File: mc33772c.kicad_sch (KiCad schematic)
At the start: 11 parts, among them U2 MC33772CTP1AE

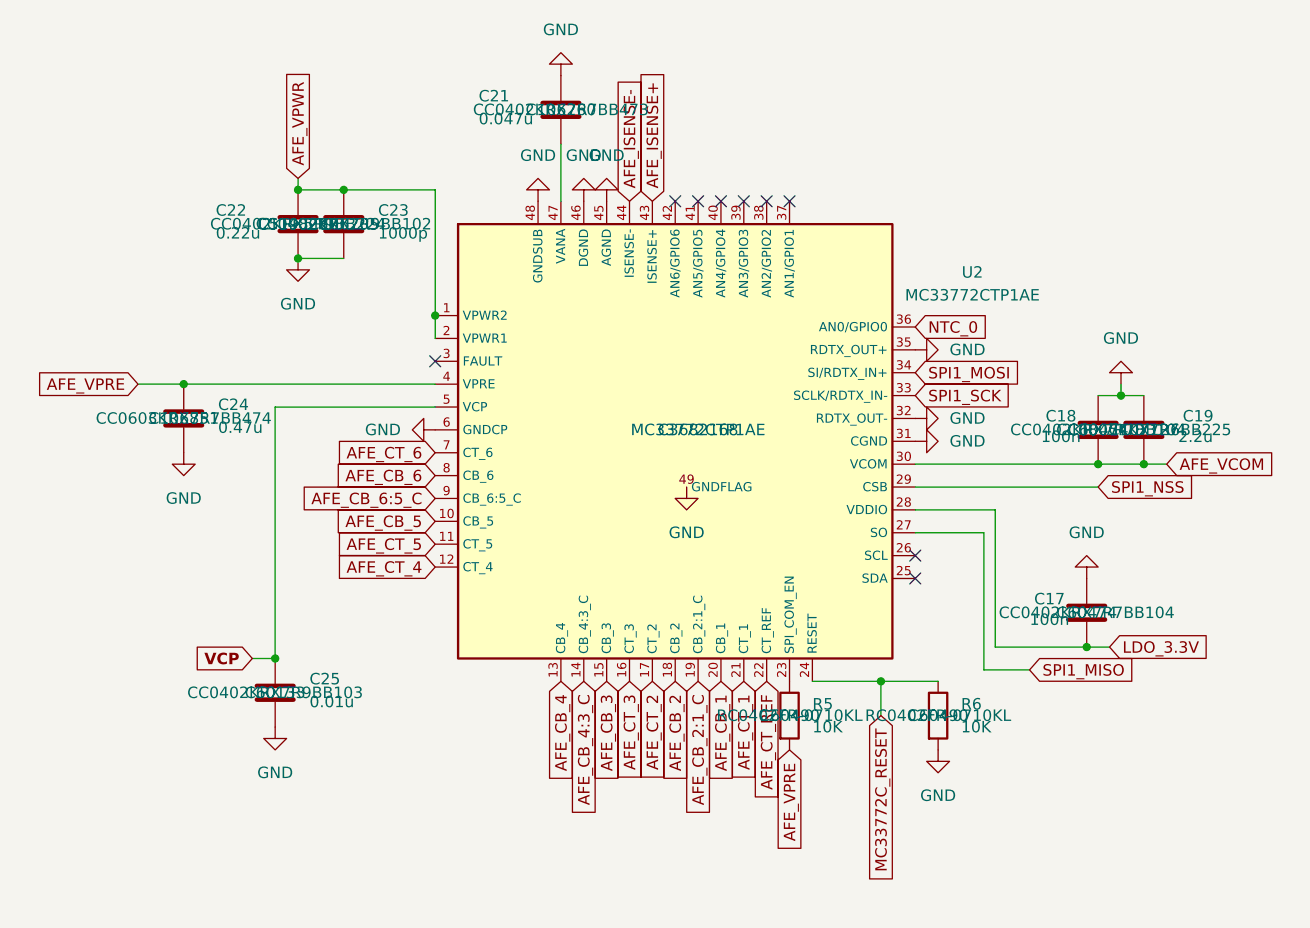
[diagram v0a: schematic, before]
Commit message: shrink, SWD
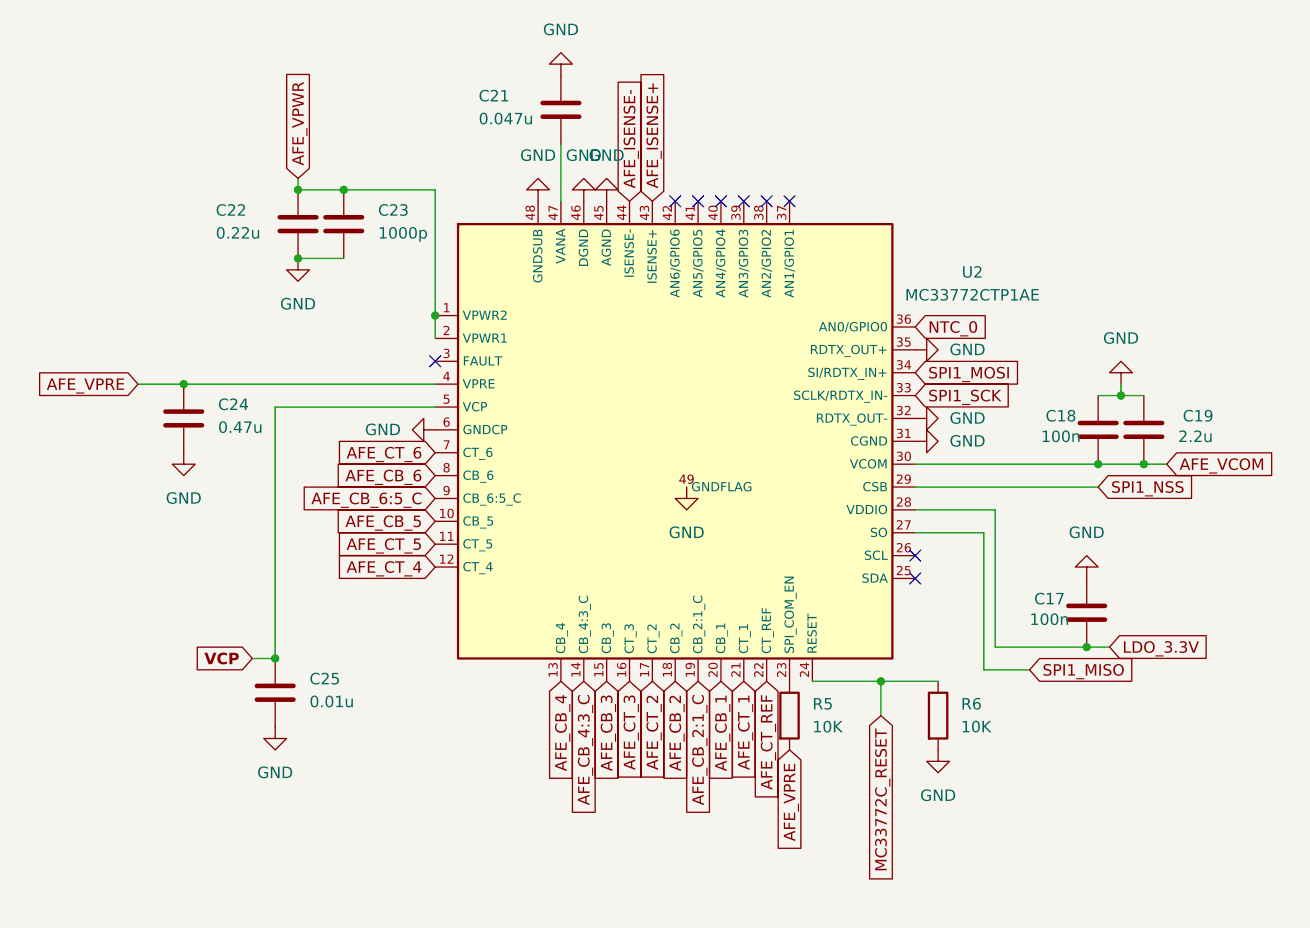
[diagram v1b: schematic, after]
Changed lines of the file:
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@@
 		(property "LCSC Part #" ""
 			(at 140.97 58.42 0)
+			(hide yes)
 			(show_name no)
 			(do_not_autoplace no)
@@
 		(property "MPN" ""
 			(at 140.97 58.42 180)
+			(hide yes)
 			(show_name no)
 			(do_not_autoplace no)
@@
 		(property "LCSC Part #" ""
 			(at 175.26 74.93 0)
+			(hide yes)
 			(show_name no)
 			(do_not_autoplace no)
@@
 		(property "MPN" ""
 			(at 175.26 74.93 90)
+			(hide yes)
 			(show_name no)
 			(do_not_autoplace no)
@@
 		(property "LCSC Part #" "C107127"
 			(at 200.66 83.82 0)
+			(hide yes)
 			(show_name no)
 			(do_not_autoplace no)
@@
 		(property "MPN" "CC0805KKX7R6BB225"
 			(at 200.66 83.82 0)
+			(hide yes)
 			(show_name no)
 			(do_not_autoplace no)
@@
 		(property "LCSC Part #" "C106851"
 			(at 93.98 82.55 0)
+			(hide yes)
 			(show_name no)
 			(do_not_autoplace no)
@@
 		(property "MPN" "CC0603KRX7R7BB474"
 			(at 93.98 82.55 0)
+			(hide yes)
 			(show_name no)
 			(do_not_autoplace no)
@@
 		(property "LCSC Part #" ""
 			(at 104.14 116.84 0)
+			(hide yes)
 			(show_name no)
 			(do_not_autoplace no)
@@
 		(property "MPN" ""
 			(at 104.14 116.84 0)
+			(hide yes)
 			(show_name no)
 			(do_not_autoplace no)
@@
 		(property "LCSC Part #" "C60490"
 			(at 177.8 115.57 0)
+			(hide yes)
 			(show_name no)
 			(do_not_autoplace no)
@@
 		(property "MPN" "RC0402FR-0710KL"
 			(at 177.8 115.57 0)
+			(hide yes)
 			(show_name no)
 			(do_not_autoplace no)
@@
 		(property "LCSC Part #" "C5198287"
 			(at 106.68 60.96 0)
+			(hide yes)
 			(show_name no)
 			(do_not_autoplace no)
@@
 		(property "MPN" "CC0402KRX5R9BB224"
 			(at 106.68 60.96 0)
+			(hide yes)
 			(show_name no)
 			(do_not_autoplace no)
@@
 		(property "LCSC Part #" "C60133"
 			(at 104.14 113.03 0)
+			(hide yes)
 			(show_name no)
 			(do_not_autoplace no)
@@
 		(property "MPN" "CC0402KRX7R9BB103"
 			(at 104.14 113.03 0)
+			(hide yes)
 			(show_name no)
 			(do_not_autoplace no)
@@
 		(property "LCSC Part #" ""
 			(at 106.68 64.77 0)
+			(hide yes)
 			(show_name no)
 			(do_not_autoplace no)
@@
 		(property "MPN" ""
 			(at 106.68 64.77 0)
+			(hide yes)
 			(show_name no)
 			(do_not_autoplace no)
@@
 		(property "LCSC Part #" "C3682168"
 			(at 151.13 83.82 0)
+			(hide yes)
 			(show_name no)
 			(do_not_autoplace no)
@@
 		(property "MPN" "MC33772CTP1AE"
 			(at 151.13 83.82 0)
+			(hide yes)
 			(show_name no)
 			(do_not_autoplace no)
@@
 		(property "LCSC Part #" ""
 			(at 175.26 85.09 0)
+			(hide yes)
 			(show_name no)
 			(do_not_autoplace no)
@@
 		(property "MPN" ""
 			(at 175.26 85.09 90)
+			(hide yes)
 			(show_name no)
 			(do_not_autoplace no)
@@
 		(property "LCSC Part #" "C60474"
 			(at 195.58 83.82 0)
+			(hide yes)
 			(show_name no)
 			(do_not_autoplace no)
@@
 		(property "MPN" "CC0402KRX7R7BB104"
 			(at 195.58 83.82 0)
+			(hide yes)
 			(show_name no)
 			(do_not_autoplace no)
@@
 		(property "LCSC Part #" ""
 			(at 175.26 82.55 0)
+			(hide yes)
 			(show_name no)
 			(do_not_autoplace no)
@@
 		(property "MPN" ""
 			(at 175.26 82.55 90)
+			(hide yes)
 			(show_name no)
 			(do_not_autoplace no)
@@
 		(property "LCSC Part #" ""
 			(at 133.35 58.42 0)
+			(hide yes)
 			(show_name no)
 			(do_not_autoplace no)
@@
 		(property "MPN" ""
 			(at 133.35 58.42 180)
+			(hide yes)
 			(show_name no)
 			(do_not_autoplace no)
@@
 		(property "LCSC Part #" ""
 			(at 194.31 100.33 0)
+			(hide yes)
 			(show_name no)
 			(do_not_autoplace no)
@@
 		(property "MPN" ""
 			(at 194.31 100.33 180)
+			(hide yes)
 			(show_name no)
 			(do_not_autoplace no)
@@
 		(property "LCSC Part #" ""
 			(at 149.86 90.17 0)
+			(hide yes)
 			(show_name no)
 			(do_not_autoplace no)
@@
 		(property "MPN" ""
 			(at 149.86 90.17 0)
+			(hide yes)
 			(show_name no)
 			(do_not_autoplace no)
@@
 		(property "LCSC Part #" ""
 			(at 138.43 58.42 0)
+			(hide yes)
 			(show_name no)
 			(do_not_autoplace no)
@@
 		(property "MPN" ""
 			(at 138.43 58.42 180)
+			(hide yes)
 			(show_name no)
 			(do_not_autoplace no)
@@
 		(property "LCSC Part #" "C60474"
 			(at 194.31 104.14 0)
+			(hide yes)
 			(show_name no)
 			(do_not_autoplace no)
@@
 		(property "MPN" "CC0402KRX7R7BB104"
 			(at 194.31 104.14 0)
+			(hide yes)
 			(show_name no)
 			(do_not_autoplace no)
@@
 		(property "LCSC Part #" ""
 			(at 121.92 83.82 0)
+			(hide yes)
 			(show_name no)
 			(do_not_autoplace no)
@@
 		(property "MPN" ""
 			(at 121.92 83.82 270)
+			(hide yes)
 			(show_name no)
 			(do_not_autoplace no)
@@
 		(property "LCSC Part #" "C106205"
 			(at 111.76 60.96 0)
+			(hide yes)
 			(show_name no)
 			(do_not_autoplace no)
@@
 		(property "MPN" "CC0402KRX7R9BB102"
 			(at 111.76 60.96 0)
+			(hide yes)
 			(show_name no)
 			(do_not_autoplace no)
@@
 		(property "LCSC Part #" ""
 			(at 93.98 86.36 0)
+			(hide yes)
 			(show_name no)
 			(do_not_autoplace no)
@@
 		(property "MPN" ""
 			(at 93.98 86.36 0)
+			(hide yes)
 			(show_name no)
 			(do_not_autoplace no)
@@
 		(property "LCSC Part #" ""
 			(at 177.8 119.38 0)
+			(hide yes)
 			(show_name no)
 			(do_not_autoplace no)
@@
 		(property "MPN" ""
 			(at 177.8 119.38 0)
+			(hide yes)
 			(show_name no)
 			(do_not_autoplace no)
@@
 		(property "LCSC Part #" ""
 			(at 135.89 44.45 0)
+			(hide yes)
 			(show_name no)
 			(do_not_autoplace no)
@@
 		(property "MPN" ""
 			(at 135.89 44.45 180)
+			(hide yes)
 			(show_name no)
 			(do_not_autoplace no)
@@
 		(property "LCSC Part #" "C60490"
 			(at 161.29 115.57 0)
+			(hide yes)
 			(show_name no)
 			(do_not_autoplace no)
@@
 		(property "MPN" "RC0402FR-0710KL"
 			(at 161.29 115.57 0)
+			(hide yes)
 			(show_name no)
 			(do_not_autoplace no)
@@
 		(property "LCSC Part #" ""
 			(at 198.12 78.74 0)
+			(hide yes)
 			(show_name no)
 			(do_not_autoplace no)
@@
 		(property "MPN" ""
 			(at 198.12 78.74 180)
+			(hide yes)
 			(show_name no)
 			(do_not_autoplace no)
@@
 		(property "LCSC Part #" "C106260"
 			(at 135.89 48.26 0)
+			(hide yes)
 			(show_name no)
 			(do_not_autoplace no)
@@
 		(property "MPN" "CC0402KRX7R7BB473"
 			(at 135.89 48.26 0)
+			(hide yes)
 			(show_name no)
 			(do_not_autoplace no)
